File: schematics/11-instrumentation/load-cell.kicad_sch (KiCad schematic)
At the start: 12 parts, among them IC1 HX711, Q1 S8550

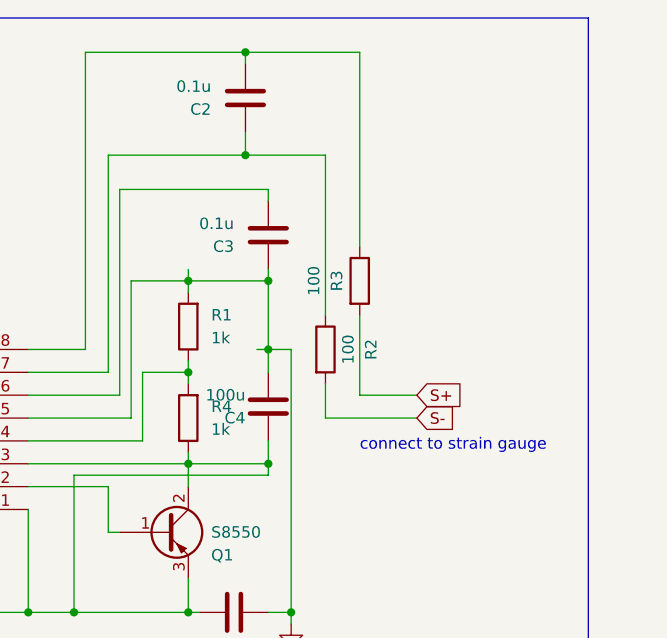
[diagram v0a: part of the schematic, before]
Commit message: load cell
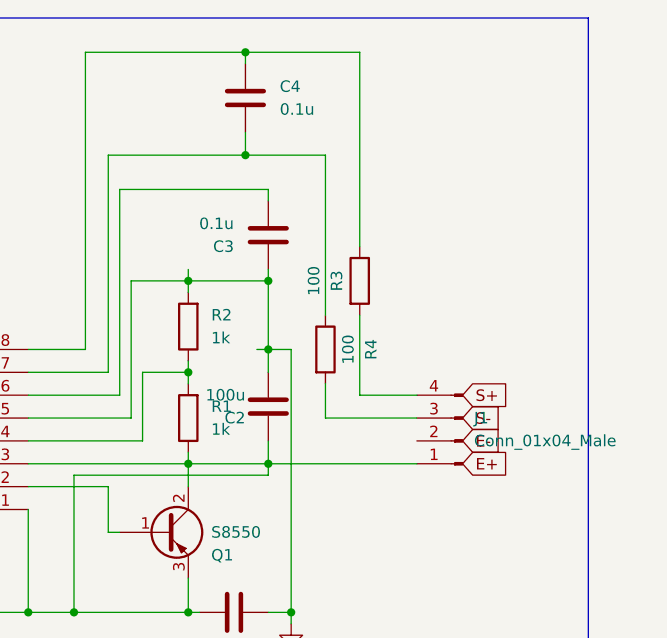
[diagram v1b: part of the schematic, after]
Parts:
- added J1: Conn_01x04_Male, symbol Connector:Conn_01x04_Male
- IC1: symbol HX711:HX711 -> royale:HX711
- renumbered C4 to C2, C2 to C4, R4 to R1, R1 to R2, R2 to R4
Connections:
- net 1v8: now also J1.1 (Pin_1)
- net S+: no longer R3.2
- net S-: no longer R4.2
- new net: J1.3 (Pin_3), R4.2
- new net: J1.4 (Pin_4), R3.2
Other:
- note removed: "connect to strain gauge"
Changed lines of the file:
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@@
+    (stroke (width 0) (type default) (color 0 0 0 0))
+  )
+  (wire (pts (xy 185.42 91.44) (xy 195.58 91.44))
     (stroke (width 0) (type default) (color 0 0 0 0))
   )
@@
     (stroke (width 0) (type default) (color 0 0 0 0))
   )
-  (wire (pts (xy 185.42 91.44) (xy 195.58 91.44))
-    (stroke (width 0) (type default) (color 0 0 0 0))
-  )
   (polyline (pts (xy 214.63 123.19) (xy 214.63 46.99))
     (stroke (width 0) (type default) (color 0 0 0 0))
@@
     (stroke (width 0) (type default) (color 0 0 0 0))
   )
+  (wire (pts (xy 189.23 88.9) (xy 195.58 88.9))
+    (stroke (width 0) (type default) (color 0 0 0 0))
+  )
   (wire (pts (xy 113.03 99.06) (xy 113.03 96.52))
     (stroke (width 0) (type default) (color 0 0 0 0))
@@
     (stroke (width 0) (type default) (color 0 0 0 0))
   )
-  (wire (pts (xy 189.23 88.9) (xy 195.58 88.9))
-    (stroke (width 0) (type default) (color 0 0 0 0))
-  )
   (wire (pts (xy 121.92 86.36) (xy 113.03 86.36))
     (stroke (width 0) (type default) (color 0 0 0 0))
@@
   )
   (wire (pts (xy 109.22 113.03) (xy 119.38 113.03))
+    (stroke (width 0) (type default) (color 0 0 0 0))
+  )
+  (wire (pts (xy 179.07 96.52) (xy 195.58 96.52))
     (stroke (width 0) (type default) (color 0 0 0 0))
   )
@@
     (effects (font (size 1.27 1.27)) (justify right bottom))
   )
-  (text "connect to strain gauge" (at 189.23 95.25 0)
-    (effects (font (size 1.27 1.27)) (justify left bottom))
-  )
   (text "Pull-Ups" (at 100.33 118.11 180)
     (effects (font (size 1.27 1.27)) (justify right bottom))
   )
-  (global_label "S-" (shape input) (at 195.58 91.44 0) (fields_autoplaced)
+  (global_label "E+" (shape input) (at 200.66 96.52 0) (fields_autoplaced)
     (effects (font (size 1.27 1.27)) (justify left))
-    (property "Intersheet References" "${INTERSHEET_REFS}" (id 0) (at 200.775 91.3606 0)
-      (effects (font (size 1.27 1.27)) (justify left) hide)
-    )
-  )
-  (global_label "S+" (shape input) (at 195.58 88.9 0) (fields_autoplaced)
+    (property "Intersheet References" "${INTERSHEET_REFS}" (id 0) (at 205.7945 96.4406 0)
+      (effects (font (size 1.27 1.27)) (justify left) hide)
+    )
+  )
+  (global_label "S-" (shape input) (at 200.66 91.44 0) (fields_autoplaced)
     (effects (font (size 1.27 1.27)) (justify left))
-    (property "Intersheet References" "${INTERSHEET_REFS}" (id 0) (at 200.775 88.8206 0)
+    (property "Intersheet References" "${INTERSHEET_REFS}" (id 0) (at 205.855 91.3606 0)
+      (effects (font (size 1.27 1.27)) (justify left) hide)
+    )
+  )
+  (global_label "E-" (shape input) (at 200.66 93.98 0) (fields_autoplaced)
+    (effects (font (size 1.27 1.27)) (justify left))
+    (property "Intersheet References" "${INTERSHEET_REFS}" (id 0) (at 205.7945 93.9006 0)
+      (effects (font (size 1.27 1.27)) (justify left) hide)
+    )
+  )
+  (global_label "S+" (shape input) (at 200.66 88.9 0) (fields_autoplaced)
+    (effects (font (size 1.27 1.27)) (justify left))
+    (property "Intersheet References" "${INTERSHEET_REFS}" (id 0) (at 205.855 88.8206 0)
       (effects (font (size 1.27 1.27)) (justify left) hide)
     )
@@
   (symbol (lib_id "Device:C") (at 179.07 90.17 180) (unit 1)
     (in_bom yes) (on_board yes)
-    (property "Reference" "C4" (id 0) (at 176.53 91.44 0)
+    (property "Reference" "C2" (id 0) (at 176.53 91.44 0)
       (effects (font (size 1.27 1.27)) (justify left))
     )
@@
     (pin "1")
   )
+  (symbol (lib_id "Connector:Conn_01x04_Male") (at 200.66 93.98 180) (unit 1)
+    (in_bom yes) (on_board yes) (fields_autoplaced)
+    (property "Reference" "J1" (id 0) (at 201.93 91.4399 0)
+      (effects (font (size 1.27 1.27)) (justify right))
+    )
+    (property "Value" "Conn_01x04_Male" (id 1) (at 201.93 93.9799 0)
+      (effects (font (size 1.27 1.27)) (justify right))
+    )
+    (property "Footprint" "" (id 2) (at 200.66 93.98 0)
+      (effects (font (size 1.27 1.27)) hide)
+    )
+    (property "Datasheet" "~" (id 3) (at 200.66 93.98 0)
+      (effects (font (size 1.27 1.27)) hide)
+    )
+    (pin "1")
+    (pin "2")
+    (pin "3")
+    (pin "4")
+  )
   (symbol (lib_id "power:GND") (at 181.61 114.3 0) (unit 1)
     (in_bom yes) (on_board yes) (fields_autoplaced)
@@
     (pin "2")
   )
-  (symbol (lib_id "HX711:HX711") (at 152.4 101.6 180) (unit 1)
+  (symbol (lib_id "royale:HX711") (at 152.4 101.6 180) (unit 1)
     (in_bom yes) (on_board yes) (fields_autoplaced)
     (property "Reference" "IC1" (id 0) (at 137.16 76.2 0))
@@
   (symbol (lib_id "Device:C") (at 176.53 55.88 180) (unit 1)
     (in_bom yes) (on_board yes) (fields_autoplaced)
-    (property "Reference" "C2" (id 0) (at 172.72 57.1501 0)
-      (effects (font (size 1.27 1.27)) (justify left))
-    )
-    (property "Value" "0.1u" (id 1) (at 172.72 54.6101 0)
-      (effects (font (size 1.27 1.27)) (justify left))
+    (property "Reference" "C4" (id 0) (at 180.34 54.6099 0)
+      (effects (font (size 1.27 1.27)) (justify right))
+    )
+    (property "Value" "0.1u" (id 1) (at 180.34 57.1499 0)
+      (effects (font (size 1.27 1.27)) (justify right))
     )
     (property "Footprint" "royale:C_0402_1005Metric_Pad0.74x0.62mm_HandSolder" (id 2) (at 175.5648 52.07 0)
@@
   (symbol (lib_id "Device:R") (at 170.18 91.44 180) (unit 1)
     (in_bom yes) (on_board yes)
-    (property "Reference" "R4" (id 0) (at 172.72 90.1699 0)
+    (property "Reference" "R1" (id 0) (at 172.72 90.1699 0)
       (effects (font (size 1.27 1.27)) (justify right))
     )
@@
   (symbol (lib_id "Device:R") (at 170.18 81.28 180) (unit 1)
     (in_bom yes) (on_board yes) (fields_autoplaced)
-    (property "Reference" "R1" (id 0) (at 172.72 80.0099 0)
+    (property "Reference" "R2" (id 0) (at 172.72 80.0099 0)
       (effects (font (size 1.27 1.27)) (justify right))
     )
@@
   (symbol (lib_id "Device:R") (at 185.42 83.82 0) (unit 1)
     (in_bom yes) (on_board yes)
-    (property "Reference" "R2" (id 0) (at 190.5 83.82 90))
+    (property "Reference" "R4" (id 0) (at 190.5 83.82 90))
     (property "Value" "100" (id 1) (at 187.96 83.82 90))
     (property "Footprint" "royale:R_0402_1005Metric_Pad0.72x0.64mm_HandSolder" (id 2) (at 183.642 83.82 90)
@@
       (reference "C1") (unit 1) (value "10u") (footprint "royale:C_0402_1005Metric_Pad0.74x0.62mm_HandSolder")
     )
-    (path "/d82854f8-978b-4c32-9d4b-da5e6d4de9ec"
-      (reference "C2") (unit 1) (value "0.1u") (footprint "royale:C_0402_1005Metric_Pad0.74x0.62mm_HandSolder")
+    (path "/36776052-bc85-446c-9b44-47290a9abc9f"
+      (reference "C2") (unit 1) (value "100u") (footprint "royale:C_0402_1005Metric_Pad0.74x0.62mm_HandSolder")
     )
     (path "/3d0f2f77-1de1-4f89-8f9a-bc30dd32b34b"
       (reference "C3") (unit 1) (value "0.1u") (footprint "royale:C_0402_1005Metric_Pad0.74x0.62mm_HandSolder")
     )
-    (path "/36776052-bc85-446c-9b44-47290a9abc9f"
-      (reference "C4") (unit 1) (value "100u") (footprint "royale:C_0402_1005Metric_Pad0.74x0.62mm_HandSolder")
+    (path "/d82854f8-978b-4c32-9d4b-da5e6d4de9ec"
+      (reference "C4") (unit 1) (value "0.1u") (footprint "royale:C_0402_1005Metric_Pad0.74x0.62mm_HandSolder")
     )
     (path "/ab488037-0bdc-49ef-a068-f0a9c636318a"
       (reference "IC1") (unit 1) (value "HX711") (footprint "hx711:SOIC127P600X160-16N")
     )
+    (path "/8e66bd57-1c49-476b-9c33-8386fa0d1d14"
+      (reference "J1") (unit 1) (value "Conn_01x04_Male") (footprint "")
+    )
     (path "/b799addf-6933-4c44-bf61-27973e36aa81"
       (reference "Q1") (unit 1) (value "S8550") (footprint "s8850:MJE13001TP")
     )
+    (path "/d91d914d-cd2d-4fe2-b31b-1921e7526d9c"
+      (reference "R1") (unit 1) (value "1k") (footprint "royale:R_0402_1005Metric_Pad0.72x0.64mm_HandSolder")
+    )
     (path "/da162b48-30bb-4fb8-b49b-4597c43d34c7"
-      (reference "R1") (unit 1) (value "1k") (footprint "royale:R_0402_1005Metric_Pad0.72x0.64mm_HandSolder")
-    )
-    (path "/e23a3038-169d-44ac-a06a-b2ed0b90cdbb"
-      (reference "R2") (unit 1) (value "100") (footprint "royale:R_0402_1005Metric_Pad0.72x0.64mm_HandSolder")
+      (reference "R2") (unit 1) (value "1k") (footprint "royale:R_0402_1005Metric_Pad0.72x0.64mm_HandSolder")
     )
     (path "/917c77a4-2bcc-4569-a027-3087491fca76"
       (reference "R3") (unit 1) (value "100") (footprint "royale:R_0402_1005Metric_Pad0.72x0.64mm_HandSolder")
     )
-    (path "/d91d914d-cd2d-4fe2-b31b-1921e7526d9c"
-      (reference "R4") (unit 1) (value "1k") (footprint "royale:R_0402_1005Metric_Pad0.72x0.64mm_HandSolder")
+    (path "/e23a3038-169d-44ac-a06a-b2ed0b90cdbb"
+      (reference "R4") (unit 1) (value "100") (footprint "royale:R_0402_1005Metric_Pad0.72x0.64mm_HandSolder")
     )
     (path "/00000000-0000-0000-0000-000062708e6f"
